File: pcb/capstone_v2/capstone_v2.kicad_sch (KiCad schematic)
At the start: 19 parts, among them IC1 HSFPAR004A, J10 NCS, J11 NCS, J13 NCS, J14 NCS, J2 VDDA, J3 VDD, J4 VDDIO, J5 GPIO, J6 INT, J7 MISO, J8 MOSI, J9 SCLK

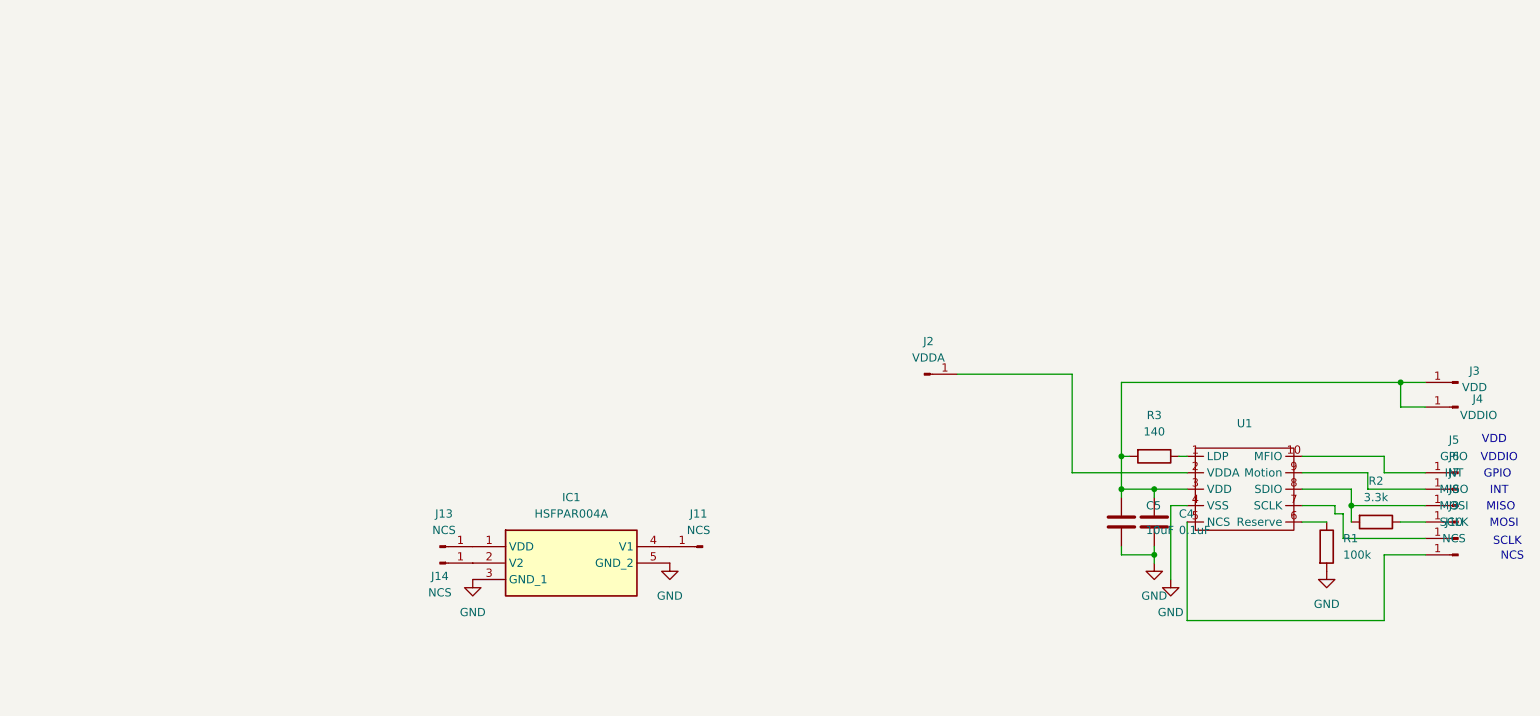
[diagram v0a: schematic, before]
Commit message: sensor and mcu board nearly complete
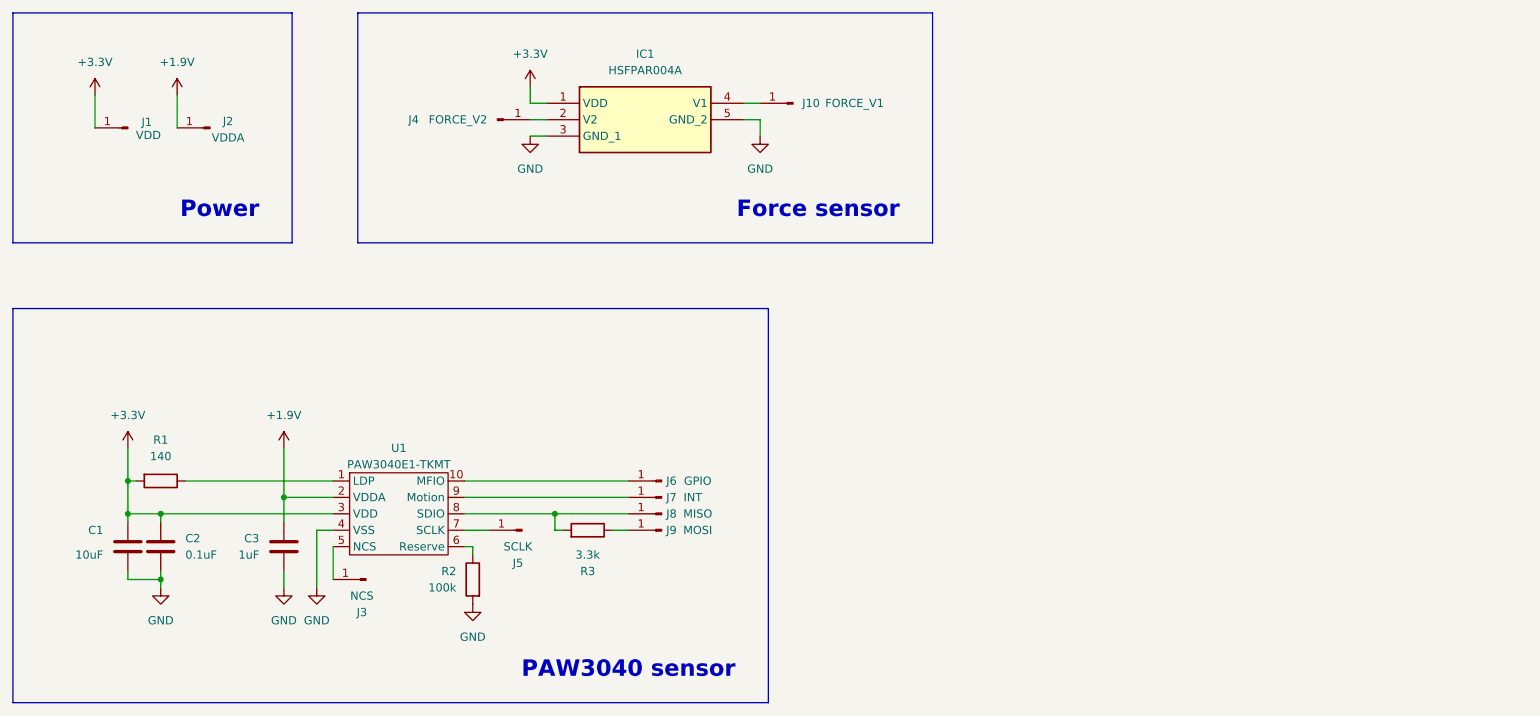
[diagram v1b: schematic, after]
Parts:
- removed J13: NCS, Connector_PinHeader_1.00mm:PinHeader_1x01_P1.00mm_Vertical, symbol Connector:Conn_01x01_Pin
- removed J4: VDDIO, Connector_PinHeader_1.00mm:PinHeader_1x01_P1.00mm_Vertical, symbol Connector:Conn_01x01_Pin
- removed U1: ~, Library:Optical_Sensor, symbol New_Library:Optical_Sensor
- added C3: 1uF, Capacitor_SMD:C_0603_1608Metric, symbol Device:C
- added U1: PAW3040E1-TKMT, Imported_FP:PAW3040E1-TKMT, symbol Custom_sym:PAW3040E1-TKMT
- C1: renamed from C5; footprint Library:CAP_CL21_SAM -> Capacitor_SMD:C_0805_2012Metric
- C2: renamed from C4; footprint Library:CAP_CL05_SAM -> Capacitor_SMD:C_0402_1005Metric
- IC1: footprint Library:HSFPAR004A -> Imported_FP:HSFPAR004A
- J10: renamed from J11; value NCS -> FORCE_V1
- J4: renamed from J14; value NCS -> FORCE_V2
- R1: renamed from R3; footprint Library:RC0603N_PAN -> Resistor_SMD:R_0603_1608Metric
- R2: renamed from R1; footprint Library:RC0603N_PAN -> Resistor_SMD:R_0603_1608Metric
- R3: renamed from R2; footprint Library:RC0603N_PAN -> Resistor_SMD:R_0402_1005Metric
- renumbered J3 to J1, J10 to J3, J9 to J5, J5 to J6, J6 to J7, J7 to J8, J8 to J9
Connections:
- net GND: now also C3.2, U1.4 (VSS)
- net +3.3V: now reaches C1.1, C2.1, J1.1 (Pin_1), R1.2
- net +3.3V: now also IC1.1 (VDD), U1.3 (VDD)
- net at J5.1 (Pin_1): now also U1.7 (SCLK)
- net at R1.1: now also U1.1 (LDP)
- net at J6.1 (Pin_1): now also U1.10 (MFIO)
- net +1.9V: now reaches J2.1 (Pin_1)
- net +1.9V: now also C3.1, U1.2 (VDDA)
- net at J3.1 (Pin_1): now also U1.5 (NCS)
- net at R2.1: now also U1.6 (Reserve)
- net at J8.1 (Pin_1), R3.2: now also U1.8 (SDIO)
- net at J7.1 (Pin_1): now also U1.9 (Motion)
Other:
- note added: "Force sensor"
- note added: "PAW3040 sensor"
- note added: "Power"
- note removed: "GPIO"
- note removed: "INT"
- note removed: "MISO"
- note removed: "MOSI"
- note removed: "NCS"
- note removed: "SCLK"
- note removed: "VDD"
- note removed: "VDDIO"
- moved on the sheet: C1, C2, IC1, J1, J10, J2, J3, J4, J5, J6, J7, J8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
